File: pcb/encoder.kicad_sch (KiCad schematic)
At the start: 18 parts, among them J17 Conn_01x04_Pin, U22 74AUP1G373, U23 74AUP1G373, U24 74LVC1G08, U25 74LVC1G08

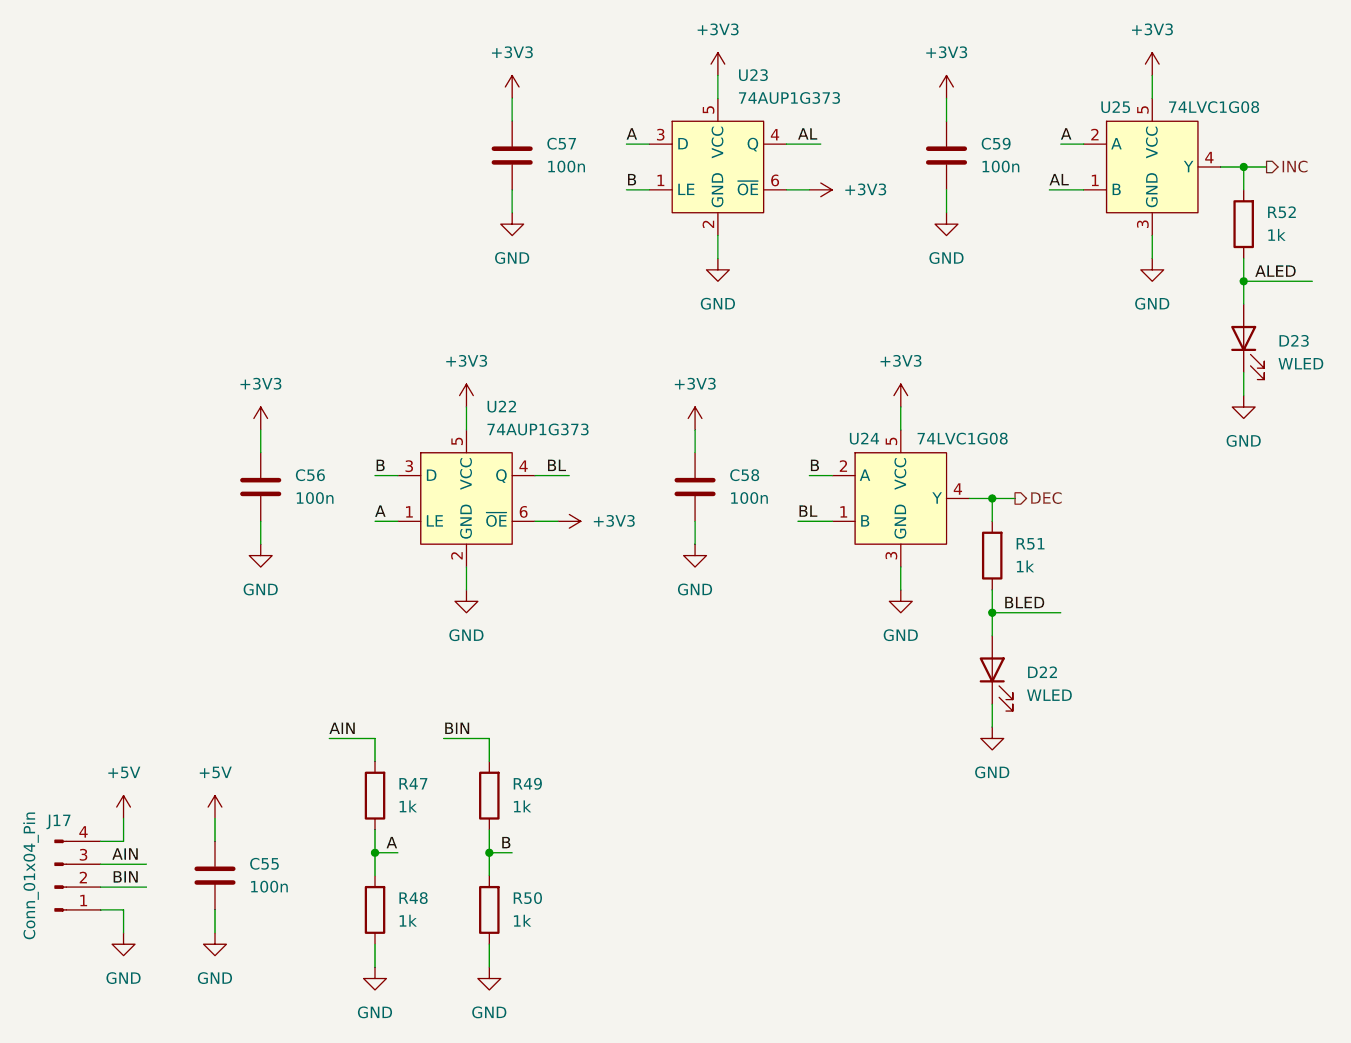
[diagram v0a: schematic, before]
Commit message: Save progress
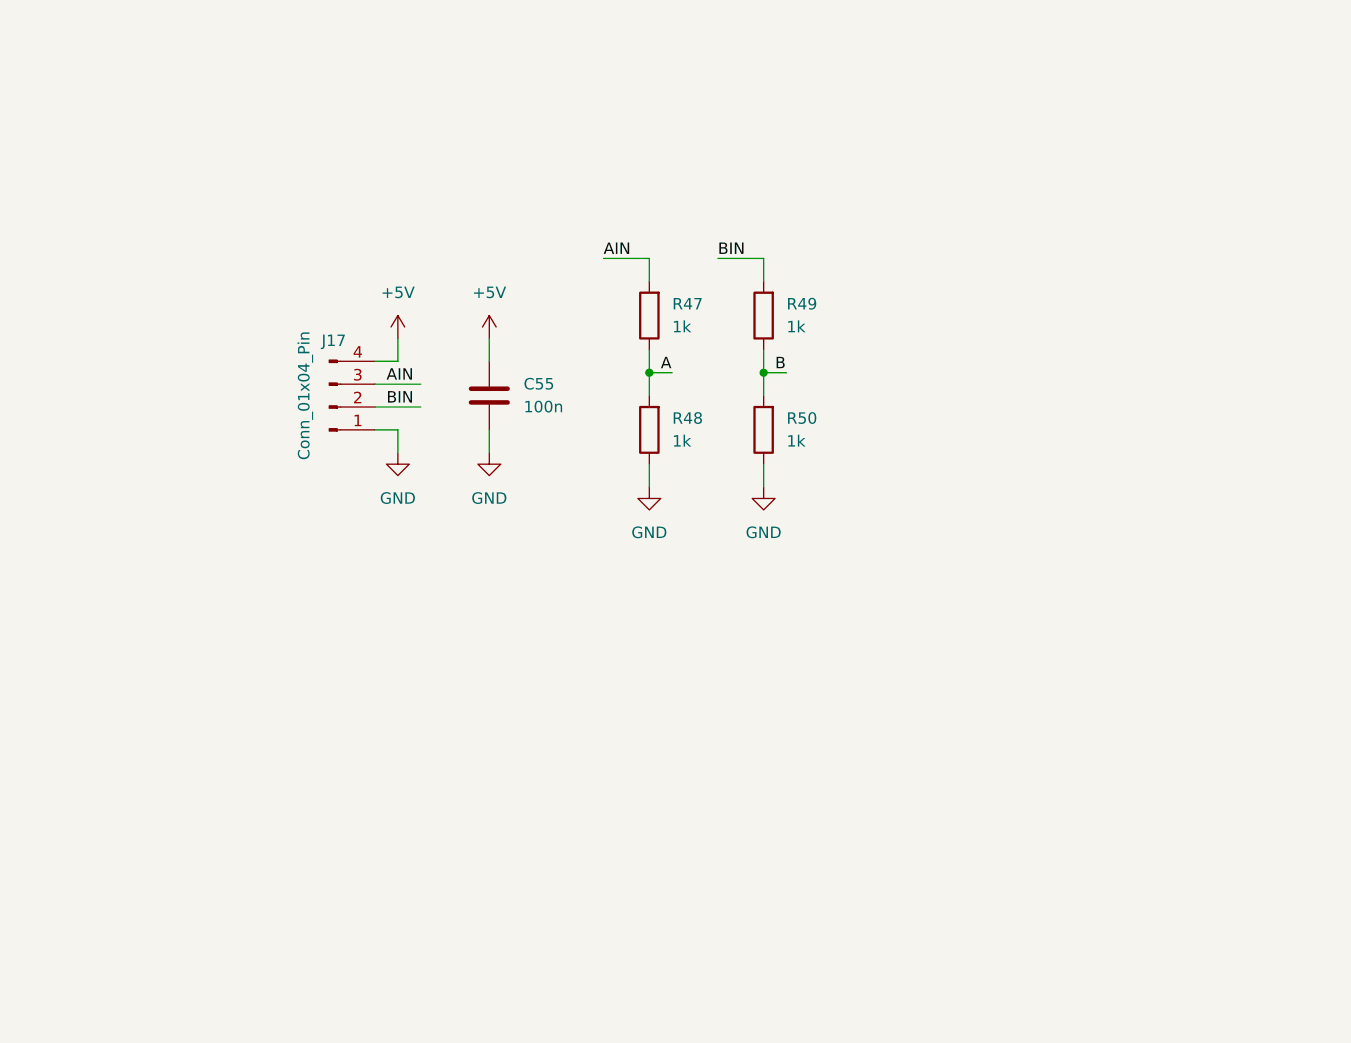
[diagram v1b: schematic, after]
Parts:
- removed C56, C57, C58, C59: 100n, Capacitor_SMD:C_0402_1005Metric, symbol Device:C
- removed D22, D23: WLED, LED_SMD:LED_0603_1608Metric, symbol Device:LED
- removed R51, R52: 1k, Resistor_SMD:R_0402_1005Metric, symbol Device:R
- removed U22, U23: 74AUP1G373, Package_TO_SOT_SMD:SOT-363_SC-70-6, symbol Symbols:74AUP1G373
- removed U24, U25: 74LVC1G08, Package_TO_SOT_SMD:SOT-353_SC-70-5, symbol Symbols:74LVC1G08
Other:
- moved on the sheet: C55, J17, R47, R48, R49, R50
